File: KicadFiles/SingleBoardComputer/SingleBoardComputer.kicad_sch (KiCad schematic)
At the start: 12 parts

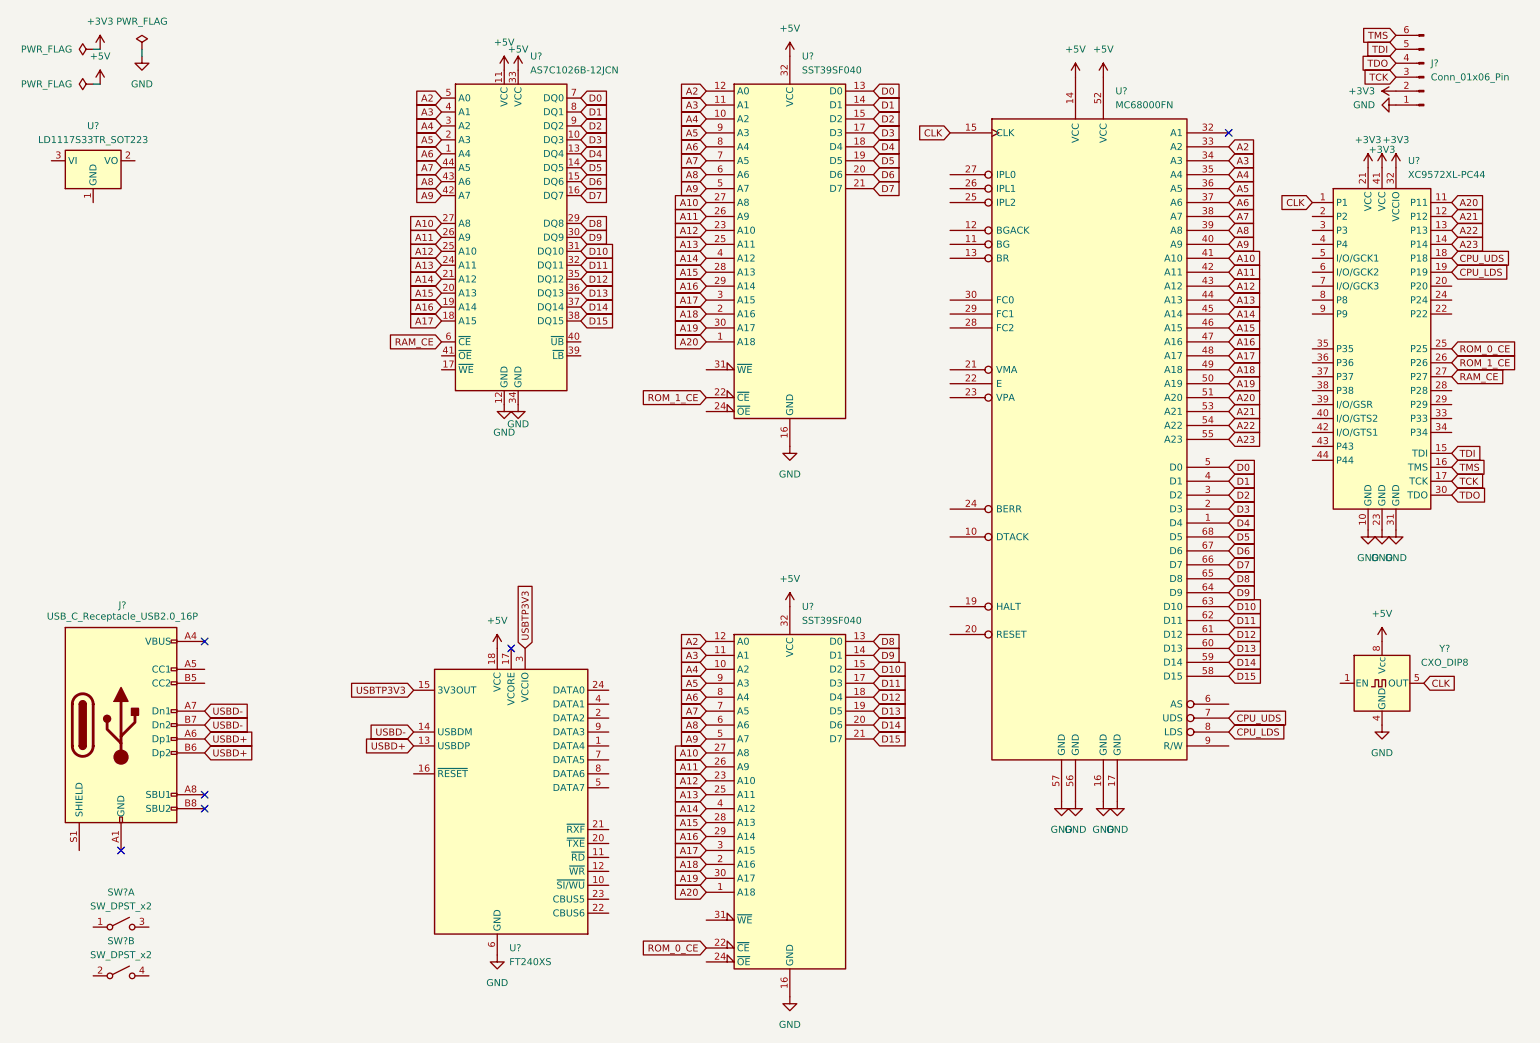
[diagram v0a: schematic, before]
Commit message: Schematic v1.0 done
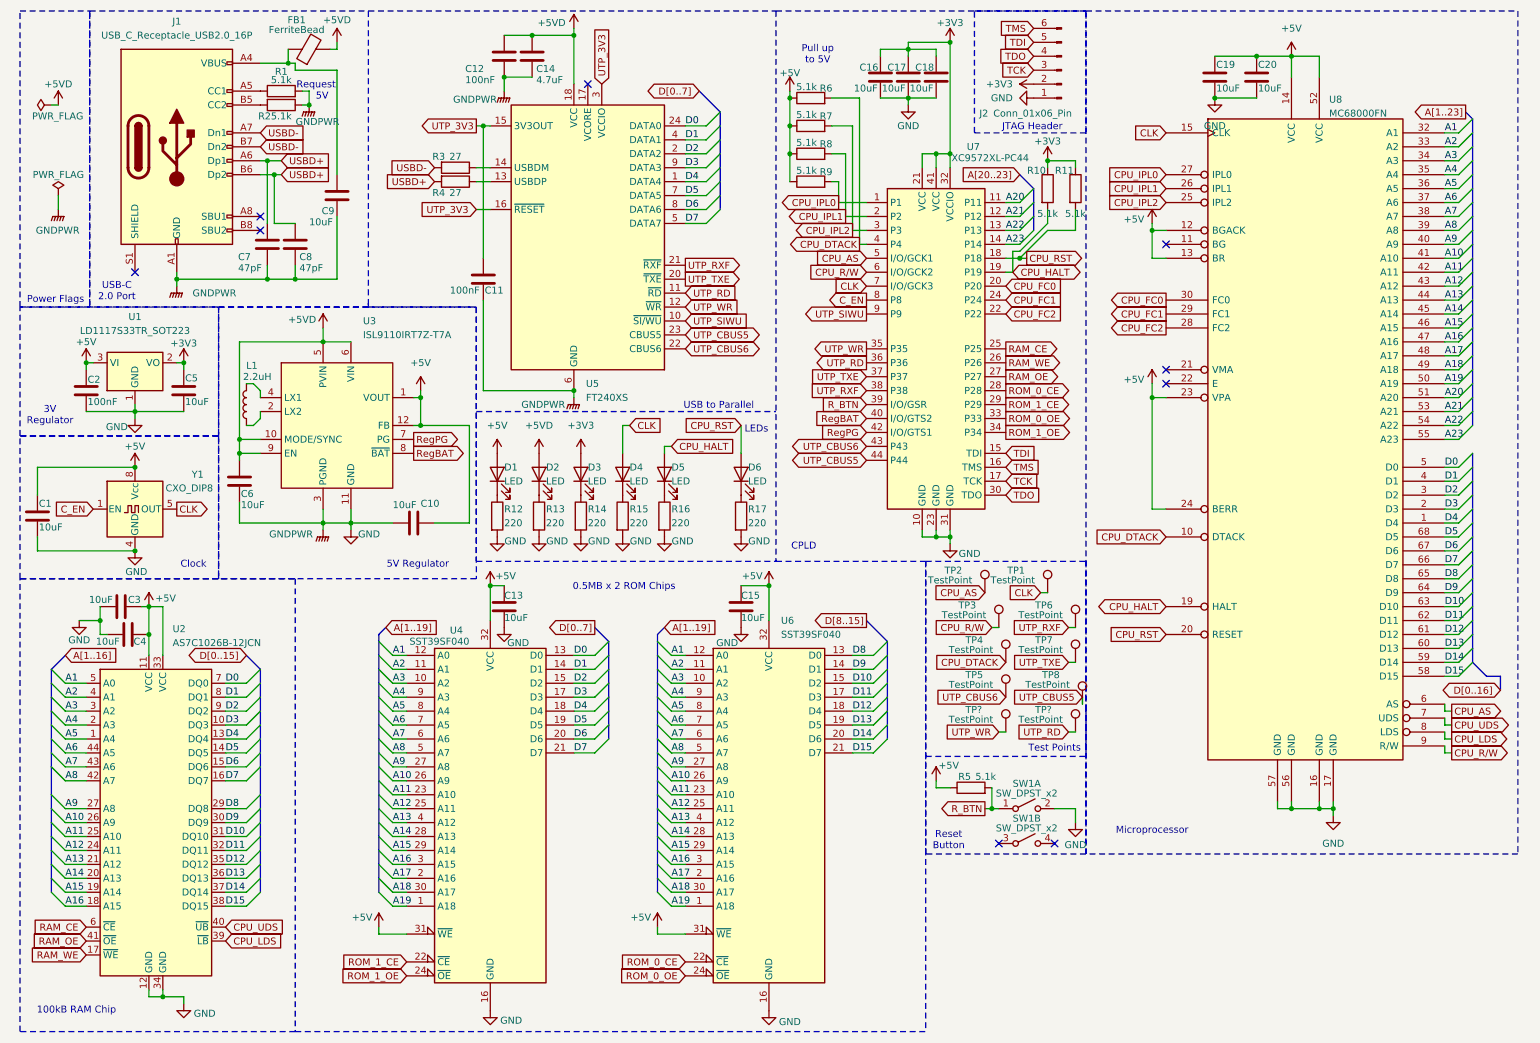
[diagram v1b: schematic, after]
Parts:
- added C1, C10, C13, C15, C16, C17, C18, C19, C20, C3, C4, C5, C6, C9: 10uF, symbol Device:C
- added C11, C12, C2: 100nF, symbol Device:C
- added C14: 4.7uF, symbol Device:C
- added C7, C8: 47pF, symbol Device:C
- added D1, D2, D3, D4, D5, D6: LED, symbol Device:LED
- added FB1: FerriteBead, symbol Device:FerriteBead
- added L1: 2.2uH, symbol Device:L
- added R1, R10, R11, R2, R5, R6, R7, R8, R9: 5.1k, symbol Device:R
- added R12, R13, R14, R15, R16, R17: 220, symbol Device:R
- added R3, R4: 27, symbol Device:R
- added TP1, TP2, TP3, TP4, TP5, TP6, TP7, TP8, TP? (x2): TestPoint, symbol Connector:TestPoint
- added U3: ISL9110IRT7Z-T7A, Package_DFN_QFN:DFN-12-1EP_3x3mm_P0.5mm_EP1.6x2.5mm_ThermalVias, symbol CustomComponents:ISL9110IRT7Z-T7A
- J1: renamed from J?; symbol Connector:USB_C_Receptacle_USB2.0_16P -> CustomComponents:USB_C_Receptacle_USB2.0_16P_Custom
- SW1: renamed from SW?; footprint (none) -> Button_Switch_SMD:SW_SPST_PTS647_Sx38
- U4, U6: renamed from U?; symbol Memory_Flash:SST39SF040 -> CustomComponents:SST39SF040_Custom
- gave numbers to parts that had none: 8
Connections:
- net USBTP3V3 is gone; now on net UTP_3V3: U5.15 (3V3OUT), U5.3 (VCCIO)
- net +3V3: now also U1.2 (VO), C16.1, C17.1, C18.1, C5.1, D3.2 (A), R10.1, R11.1
- net +5V: now also U1.3 (VI), U4.31 (~{WE}), U6.31 (~{WE}), U8.12 (BGACK), U8.13 (BR), U8.23 (VPA), U8.24 (BERR), C1.1, C10.1, C13.1, C15.1, C19.1, C2.1, C20.1, C3.1, C4.1, D1.2 (A), R5.1, R6.1, R7.1, R8.1, R9.1, U3.1 (VOUT), U3.12 (FB); no longer U5.18 (VCC)
- net A10: now also U2.26 (A9), U4.26 (A9), U6.26 (A9); no longer U2.27 (A8), U4.27 (A8), U6.27 (A8)
- net A11: now also U2.25 (A10), U4.23 (A10), U6.23 (A10); no longer U2.26 (A9), U4.26 (A9), U6.26 (A9)
- net A12: now also U2.24 (A11), U4.25 (A11), U6.25 (A11); no longer U2.25 (A10), U4.23 (A10), U6.23 (A10)
- net A13: now also U2.21 (A12), U4.4 (A12), U6.4 (A12); no longer U2.24 (A11), U4.25 (A11), U6.25 (A11)
- net A14: now also U2.20 (A13), U4.28 (A13), U6.28 (A13); no longer U2.21 (A12), U4.4 (A12), U6.4 (A12)
- net A15: now also U2.19 (A14), U4.29 (A14), U6.29 (A14); no longer U2.20 (A13), U4.28 (A13), U6.28 (A13)
- net A16: now also U2.18 (A15), U4.3 (A15), U6.3 (A15); no longer U2.19 (A14), U4.29 (A14), U6.29 (A14)
- net A17: now also U4.2 (A16), U6.2 (A16); no longer U2.18 (A15), U4.3 (A15), U6.3 (A15)
- net A18: now also U4.30 (A17), U6.30 (A17); no longer U4.2 (A16), U6.2 (A16)
- net A19: now also U4.1 (A18), U6.1 (A18); no longer U4.30 (A17), U6.30 (A17)
- net A2: now also U2.4 (A1), U4.11 (A1), U6.11 (A1); no longer U2.5 (A0), U4.12 (A0), U6.12 (A0)
- net A20: no longer U4.1 (A18), U6.1 (A18)
- net A3: now also U2.3 (A2), U4.10 (A2), U6.10 (A2); no longer U2.4 (A1), U4.11 (A1), U6.11 (A1)
- net A4: now also U2.2 (A3), U4.9 (A3), U6.9 (A3); no longer U2.3 (A2), U4.10 (A2), U6.10 (A2)
- net A5: now also U2.1 (A4), U4.8 (A4), U6.8 (A4); no longer U2.2 (A3), U4.9 (A3), U6.9 (A3)
- net A6: now also U2.44 (A5), U4.7 (A5), U6.7 (A5); no longer U2.1 (A4), U4.8 (A4), U6.8 (A4)
- net A7: now also U2.43 (A6), U4.6 (A6), U6.6 (A6); no longer U2.44 (A5), U4.7 (A5), U6.7 (A5)
- net A8: now also U2.42 (A7), U4.5 (A7), U6.5 (A7); no longer U2.43 (A6), U4.6 (A6), U6.6 (A6)
- net A9: now also U2.27 (A8), U4.27 (A8), U6.27 (A8); no longer U2.42 (A7), U4.5 (A7), U6.5 (A7)
- net CLK: now also U7.7 (I/O/GCK3), D4.2 (A), TP1.1; no longer U7.1 (P1)
- net CPU_LDS: now also U2.39 (~{LB}); no longer U7.19 (P19)
- net CPU_UDS: now also U2.40 (~{UB}); no longer U7.18 (P18)
- net D0: now also U5.24 (DATA0)
- net D1: now also U5.4 (DATA1)
- net D2: now also U5.2 (DATA2)
- net D3: now also U5.9 (DATA3)
- net D4: now also U5.1 (DATA4)
- net D5: now also U5.7 (DATA5)
- net D6: now also U5.8 (DATA6)
- net D7: now also U5.5 (DATA7)
- net GND: now also J1.A1 (GND), J1.A12 (GND), J1.B1 (GND), J1.B12 (GND), SW1.2 (B), U1.1 (GND), C1.2, C10.2, C11.2, C12.2, C13.2, C14.2, C15.2, C16.2, C17.2, C18.2, C19.2, C2.2, C20.2, C3.2, C4.2, C5.2, C6.2, C7.2, C8.2, C9.2, R1.2, R12.2, R13.2, R14.2, R15.2, R16.2, R17.2, R2.1, U3.11 (GND), U3.3 (PGND)
- net RAM_CE: now also U7.25 (P25); no longer U7.27 (P27)
- net ROM_0_CE: now also U7.28 (P28); no longer U7.25 (P25)
- net ROM_1_CE: now also U7.29 (P29); no longer U7.26 (P26)
- net USBD+: now also C7.1, C8.1, R4.2; no longer U5.13 (USBDP)
- net USBD-: now also R3.2; no longer U5.14 (USBDM)
- net UTP_SIWU: now reaches U5.10 (~{SI/WU})
- net UTP_SIWU: now also U7.9 (P9)
- net UTP_RD: now reaches U5.11 (~{RD})
- net UTP_RD: now also U7.36 (P36), TP?.1
- net UTP_WR: now reaches U5.12 (~{WR})
- net UTP_WR: now also U7.35 (P35), TP?.1
- net UTP_3V3: now reaches U5.16 (~{RESET})
- net UTP_3V3: now also C11.1
- net UTP_TXE: now reaches U5.20 (~{TXE})
- net UTP_TXE: now also U7.37 (P37), TP7.1
- net UTP_RXF: now reaches U5.21 (~{RXF})
- net UTP_RXF: now also U7.38 (P38), TP6.1
- net UTP_CBUS6: now reaches U5.22 (CBUS6)
- net UTP_CBUS6: now also U7.43 (P43), TP5.1
- net UTP_CBUS5: now reaches U5.23 (CBUS5)
- net UTP_CBUS5: now also U7.44 (P44), TP8.1
- net RAM_WE: now reaches U2.17 (~{WE})
- net RAM_WE: now also U7.26 (P26)
- net RAM_OE: now reaches U2.41 (~{OE})
- net RAM_OE: now also U7.27 (P27)
- net CPU_DTACK: now reaches U8.10 (DTACK)
- net CPU_DTACK: now also U7.4 (P4), R6.2, TP4.1
- net CPU_HALT: now reaches U8.19 (HALT)
- net CPU_HALT: now also U7.19 (P19), D5.2 (A), R10.2
- net CPU_RST: now reaches U8.20 (RESET)
- net CPU_RST: now also U7.18 (P18), D6.2 (A), R11.2
- net CPU_IPL2: now reaches U8.25 (IPL2)
- net CPU_IPL2: now also U7.3 (P3), R7.2
- net CPU_IPL1: now reaches U8.26 (IPL1)
- net CPU_IPL1: now also U7.2 (P2), R8.2
- net CPU_IPL0: now reaches U8.27 (IPL0)
- net CPU_IPL0: now also U7.1 (P1), R9.2
- net CPU_FC2: now reaches U8.28 (FC2)
- net CPU_FC2: now also U7.22 (P22)
- net CPU_FC1: now reaches U8.29 (FC1)
- net CPU_FC1: now also U7.24 (P24)
- net CPU_FC0: now reaches U8.30 (FC0)
- net CPU_FC0: now also U7.20 (P20)
- net A1: now reaches U8.32 (A1)
- net A1: now also U2.5 (A0), U4.12 (A0), U6.12 (A0)
- net CPU_AS: now reaches U8.6 (AS)
- net CPU_AS: now also U7.5 (I/O/GCK1), TP2.1
- net CPU_R/W: now reaches U8.9 (R/W)
- net CPU_R/W: now also U7.6 (I/O/GCK2), TP3.1
- net ROM_1_OE: now reaches U4.24 (~{OE})
- net ROM_1_OE: now also U7.34 (P34)
- net R_BTN: now reaches SW1.1 (A)
- net R_BTN: now also U7.39 (I/O/GSR), R5.2
- net ROM_0_OE: now reaches U6.24 (~{OE})
- net ROM_0_OE: now also U7.33 (P33)
- net RegBAT: now reaches U7.40 (I/O/GTS2)
- net RegBAT: now also U3.8 (~{BAT})
- net RegPG: now reaches U7.42 (I/O/GTS1)
- net RegPG: now also U3.7 (PG)
- net C_EN: now reaches U7.8 (P8)
- net C_EN: now also Y1.1 (EN)
- net at J1.A4 (VBUS), J1.A9 (VBUS), J1.B4 (VBUS)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: now also C9.1, FB1.1
- net at J1.A5 (CC1): now also R1.1
- net at J1.B5 (CC2): now also R2.2
- new net: D3.1 (K), R14.1
- new net: D4.1 (K), R15.1
- new net: L1.1, U3.2 (LX2)
- new net: L1.2, U3.4 (LX1)
- new net: R4.1, U5.13 (USBDP)
- new net: D5.1 (K), R16.1
- new net: D1.1 (K), R12.1
- new net: R3.1, U5.14 (USBDM)
- new net: D6.1 (K), R17.1
- new net: D2.1 (K), R13.1
- new net +5VD: C12.1, C14.1, C6.1, D2.2 (A), FB1.2, U3.10 (MODE/SYNC), U3.5 (PVIN), U3.6 (VIN), U3.9 (EN), U5.18 (VCC)
- no-connect marks 6 -> 9
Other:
- note added: "0.5MB x 2 ROM Chips"
- note added: "100kB RAM Chip"
- note added: "3V Regulator"
- note added: "5V Regulator"
- note added: "CPLD"
- note added: "Clock"
- note added: "JTAG Header"
- note added: "LEDs"
- note added: "Microprocessor"
- note added: "Power Flags"
- note added: "Pull up to 5V"
- note added: "Request 5V"
- note added: "Reset Button"
- note added: "Test Points"
- note added: "USB to Parallel"
- note added: "USB-C 2.0 Port"
- company: (none) -> Letourneau University
- title: (none) -> Single Board Computer
- moved on the sheet: J1, J2, SW1A, SW1B, U1, U2, U4, U5, U6, U7, U8, Y1

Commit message: Schematic V2.0
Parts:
- removed R10, R11, R6, R7, R8, R9: 5.1k, symbol Device:R
- added R12, R13, R14, R15, R16, R17, R18, R19, R20, R21, R22, R23, R24, R25, R26, R27, R28, R29, R30, R31, R32, R33, R34, R35: 5.1k, symbol Device:R
- gave numbers to parts that had none: 2
- renumbered C12 to C1, C8 to C10, C2 to C11, C5 to C12, C1 to C13, C16 to C14, C17 to C15, C18 to C16, C13 to C17, C15 to C18, C3 to C19, C14 to C2, C4 to C20, C19 to C3, C20 to C4, C6 to C5, C9 to C6, C11 to C7, C10 to C8, C7 to C9, R16 to R10, R17 to R11, R12 to R6, R13 to R7, R14 to R8, R15 to R9, TP2 to TP1, TP1 to TP2, TP6 to TP4, TP4 to TP5, TP7 to TP6, TP5 to TP7, U3 to U1, U5 to U2, U1 to U3, U8 to U4, U7 to U5, U4 to U6, U6 to U7, U2 to U8
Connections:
- net +5V: now also R12.1, R13.1, R14.1, R15.1, R16.1, R17.1, R18.1, R19.1, R20.1, R21.1, R22.1, R23.1, R24.1, R25.1, R26.1, R27.1, R28.1, R29.1, R30.1, R31.1, R32.1, R33.1, R34.1, R35.1
- net CPU_AS: now also R22.2
- net CPU_DTACK: now also R23.2
- net CPU_FC0: now also R29.2
- net CPU_FC1: now also R30.2
- net CPU_FC2: now also R31.2
- net CPU_HALT: now also R28.2
- net CPU_IPL0: now also R26.2
- net CPU_IPL1: now also R25.2
- net CPU_IPL2: now also R24.2
- net CPU_RST: now also R27.2
- net CPU_R/W: now also R21.2
- net C_EN: now also R20.2
- net RAM_CE: now also R12.2
- net RAM_OE: now also R14.2
- net RAM_WE: now also R13.2
- net ROM_0_CE: now also R32.2
- net ROM_0_OE: now also R34.2
- net ROM_1_CE: now also R33.2
- net ROM_1_OE: now also R35.2
- net R_BTN: now also R19.2
- net RegBAT: now also R18.2
- net RegPG: now also R17.2
- net UTP_CBUS5: now also R15.2
- net UTP_CBUS6: now also R16.2
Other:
- note added: "131kB RAM Chip"
- note removed: "100kB RAM Chip"
- moved on the sheet: C1, C10, C11, C12, C13, C14, C15, C16, C17, C18, C19, C2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
